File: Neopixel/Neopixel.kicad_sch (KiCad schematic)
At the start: 70 parts

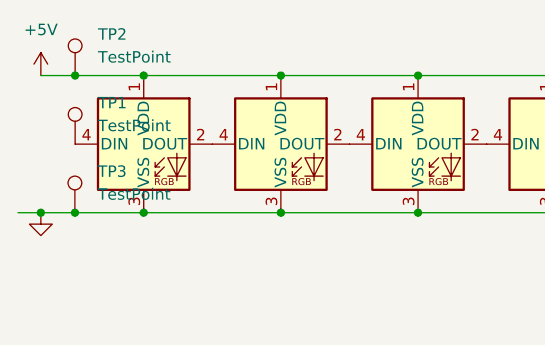
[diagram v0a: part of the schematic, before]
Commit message: designing
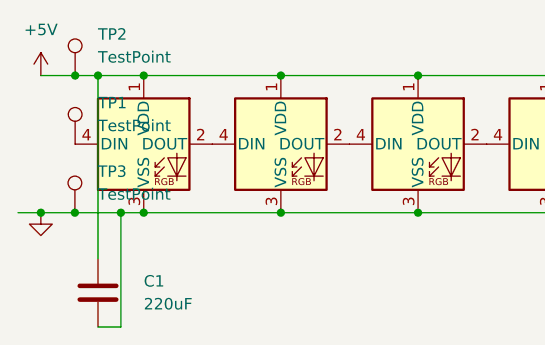
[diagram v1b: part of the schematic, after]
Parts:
- added C1: 220uF, Capacitor_SMD:C_1206_3216Metric, symbol Device:C
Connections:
- net +5V: now also C1.1
- net GND: now also C1.2
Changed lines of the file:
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@@
 	)
 	(junction
+		(at -313.69 29.21)
+		(diameter 0)
+		(color 0 0 0 0)
+	)
+	(junction
 		(at -219.71 13.97)
 		(diameter 0)
@@
 	)
 	(junction
+		(at -316.23 13.97)
+		(diameter 0)
+		(color 0 0 0 0)
+	)
+	(junction
 		(at 450.85 29.21)
 		(diameter 0)
@@
 	(wire
 		(pts
+			(xy -313.69 29.21) (xy -311.15 29.21)
+		)
+		(stroke
+			(width 0)
+			(type default)
+		)
+	)
+	(wire
+		(pts
 			(xy -325.12 29.21) (xy -322.58 29.21)
 		)
@@
 	(wire
 		(pts
-			(xy -318.77 13.97) (xy -311.15 13.97)
+			(xy -318.77 13.97) (xy -316.23 13.97)
 		)
 		(stroke
@@
 	(wire
 		(pts
-			(xy -318.7968 29.21) (xy -311.15 29.21)
+			(xy -318.7968 29.21) (xy -313.69 29.21)
 		)
 		(stroke
@@
 	(wire
 		(pts
+			(xy -316.23 13.97) (xy -311.15 13.97)
+		)
+		(stroke
+			(width 0)
+			(type default)
+		)
+	)
+	(wire
+		(pts
 			(xy -52.07 29.21) (xy -67.31 29.21)
 		)
@@
 	(wire
 		(pts
+			(xy -313.69 41.91) (xy -313.69 29.21)
+		)
+		(stroke
+			(width 0)
+			(type default)
+		)
+	)
+	(wire
+		(pts
 			(xy -6.35 29.21) (xy 8.89 29.21)
 		)
@@
 	(wire
 		(pts
+			(xy -316.23 41.91) (xy -313.69 41.91)
+		)
+		(stroke
+			(width 0)
+			(type default)
+		)
+	)
+	(wire
+		(pts
 			(xy 389.89 13.97) (xy 405.13 13.97)
 		)
@@
 	(wire
 		(pts
+			(xy -316.23 13.97) (xy -316.23 34.29)
+		)
+		(stroke
+			(width 0)
+			(type default)
+		)
+	)
+	(wire
+		(pts
 			(xy 359.41 13.97) (xy 374.65 13.97)
 		)
@@
 					(unit 1)
 				)
+			)
+		)
+	)
+	(symbol
+		(lib_id "Device:C")
+		(at -316.23 38.1 0)
+		(unit 1)
+		(exclude_from_sim no)
+		(in_bom yes)
+		(on_board yes)
+		(dnp no)
+		(fields_autoplaced yes)
+		(property "Reference" "C1"
+			(at -311.15 36.8299 0)
+			(effects
+				(font
+					(size 1.27 1.27)
+				)
+				(justify left)
+			)
+		)
+		(property "Value" "220uF"
+			(at -311.15 39.3699 0)
+			(effects
+				(font
+					(size 1.27 1.27)
+				)
+				(justify left)
+			)
+		)
+		(property "Footprint" "Capacitor_SMD:C_1206_3216Metric"
+			(at -315.2648 41.91 0)
+			(effects
+				(font
+					(size 1.27 1.27)
+				)
+				(hide yes)
+			)
+		)
+		(property "Datasheet" "~"
+			(at -316.23 38.1 0)
+			(effects
+				(font
+					(size 1.27 1.27)
+				)
+				(hide yes)
+			)
+		)
+		(property "Description" "Unpolarized capacitor"
+			(at -316.23 38.1 0)
+			(effects
+				(font
+					(size 1.27 1.27)
+				)
+				(hide yes)
+			)
+		)
+		(property "LCSC" "C412252"
+			(at -316.23 38.1 0)
+			(effects
+				(font
+					(size 1.27 1.27)
+				)
+				(hide yes)
+			)
+		)
+		(pin "2"
+		)
+		(pin "1"
+		)
+		(instances
+			(project ""
+				(path "/0c64f9f6-2337-46e9-954e-fa62cdf10650"
+					(reference "C1")
+					(unit 1)
+				)
